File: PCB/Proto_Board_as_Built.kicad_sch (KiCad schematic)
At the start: 17 parts, among them J1 RJ25, J2 RJ45, U1 Pico, U2 LM358

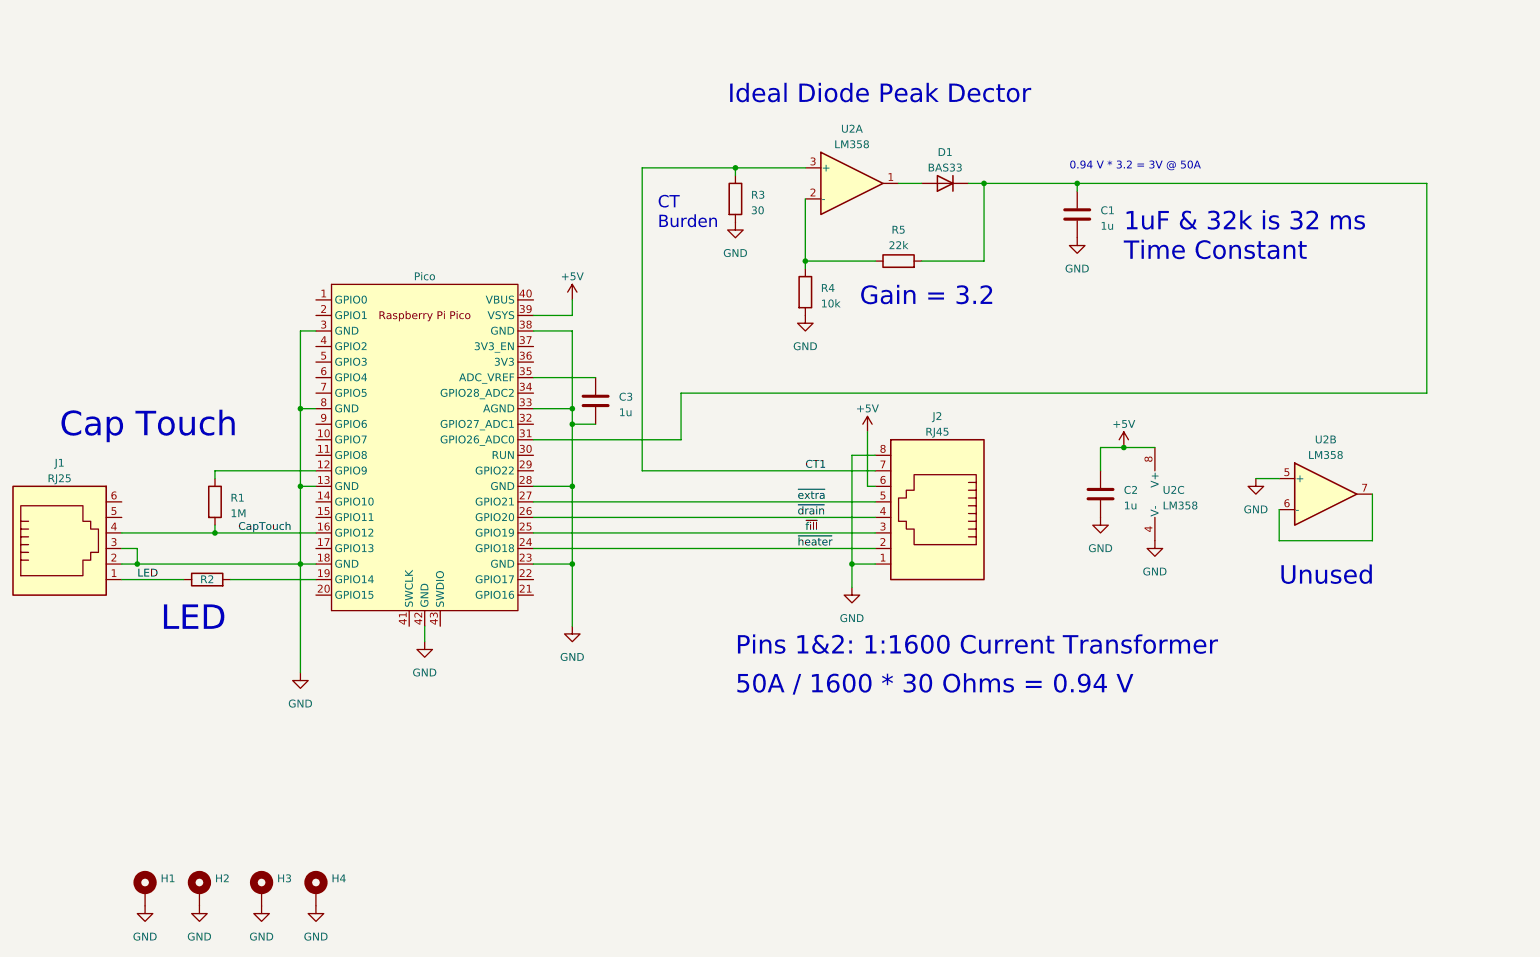
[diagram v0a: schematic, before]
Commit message: pcb updates
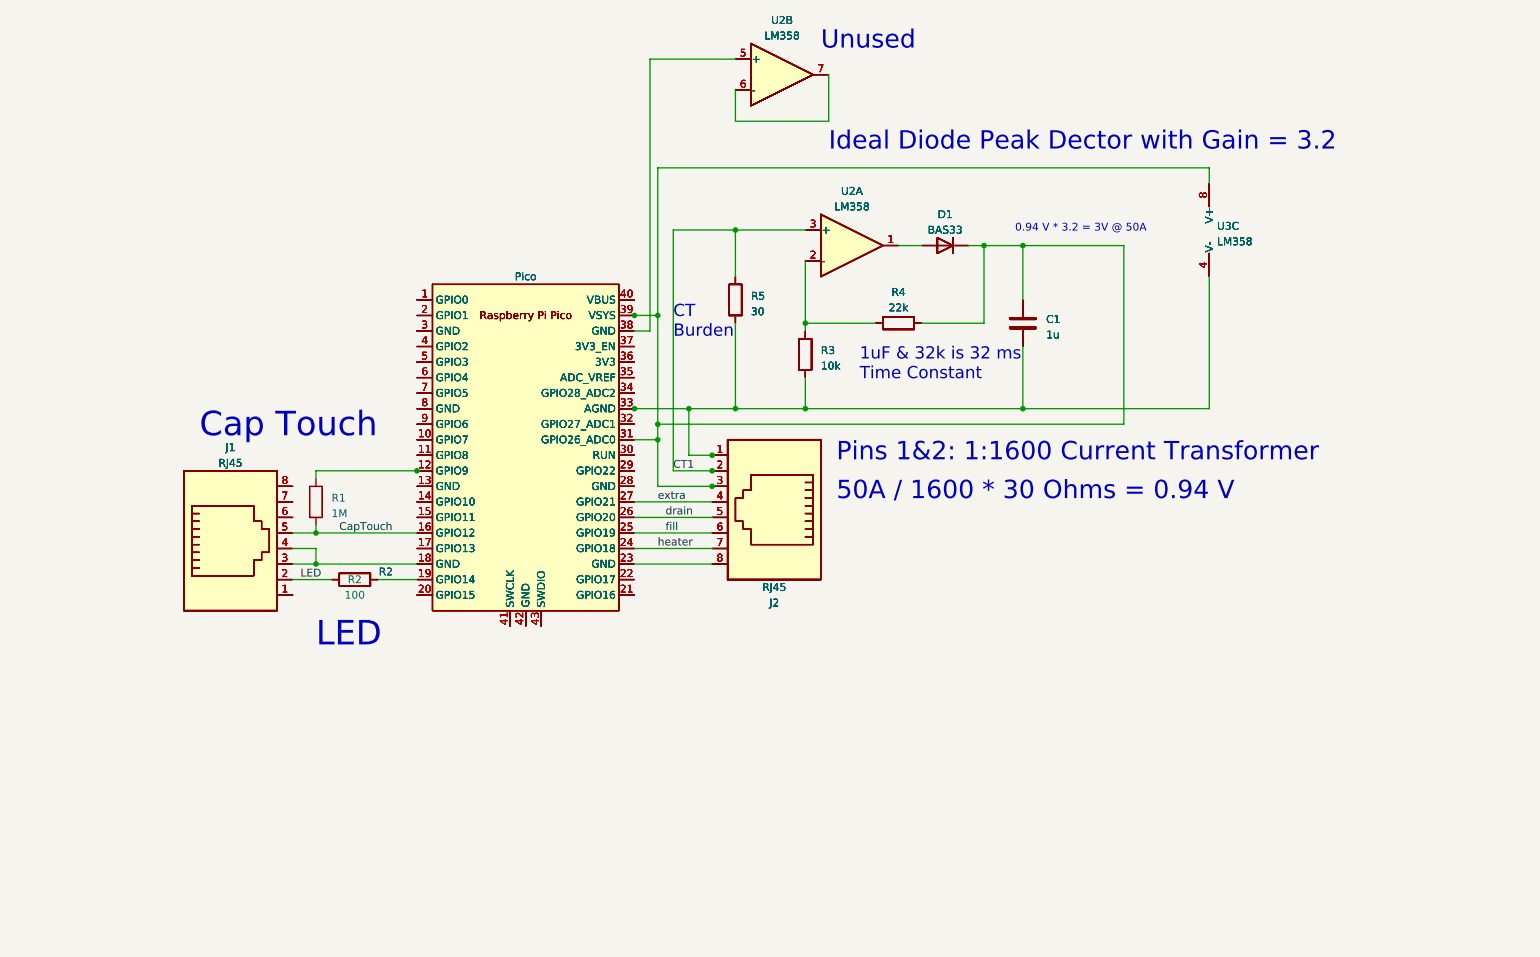
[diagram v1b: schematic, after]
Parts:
- removed C2, C3: 1u, Capacitor_SMD:C_0805_2012Metric_Pad1.18x1.45mm_HandSolder, symbol Device:C
- removed H1, H2, H3, H4: MountingHole_Pad, MountingHole:MountingHole_2.7mm_M2.5_Pad, symbol Mechanical:MountingHole_Pad
- removed J1: RJ25, Connector_RJ:RJ25_Wayconn_MJEA-660X1_Horizontal, symbol Connector:RJ25
- removed J2: RJ45, Connector_RJ:RJ45_Amphenol_54602-x08_Horizontal, symbol Connector:RJ45
- added C1 (x2): 1u, symbol Device:C
- added D1 (x2): BAS33, Diode_THT:D_DO-35_SOD27_P7.62mm_Horizontal, symbol Diode:BAV17
- added J1 (x3), J2 (x3): RJ45, symbol Connector:RJ45
- added R2 (x2): 100, symbol Device:R
- added R3 (x2): 10k, symbol Device:R
- added R4 (x2): 22k, symbol Device:R
- added R5 (x2): 30, symbol Device:R
- added U1 (x2): Pico, MCU_RaspberryPi_and_Boards:RPi_Pico_SMD_TH, symbol MCU_RaspberryPi_and_Boards:Pico
- added U2 (x2), U3 (x2): LM358, symbol Amplifier_Operational:LM358
- C1: footprint Capacitor_SMD:C_0805_2012Metric_Pad1.18x1.45mm_HandSolder -> (none)
- R1, R2: footprint Resistor_SMD:R_0805_2012Metric_Pad1.20x1.40mm_HandSolder -> (none)
- R3: renamed from R4; footprint Resistor_SMD:R_0805_2012Metric_Pad1.20x1.40mm_HandSolder -> (none)
- R4: renamed from R5; footprint Resistor_SMD:R_0805_2012Metric_Pad1.20x1.40mm_HandSolder -> (none)
- R5: renamed from R3; footprint Resistor_SMD:R_0805_2012Metric_Pad1.20x1.40mm_HandSolder -> (none)
- U1: footprint MCU_RaspberryPi_and_Boards:RPi_Pico_SMD -> MCU_RaspberryPi_and_Boards:RPi_Pico_SMD_TH
- U2: footprint Package_DIP:DIP-8_W10.16mm -> (none)
- U3: renamed from U2; footprint Package_DIP:DIP-8_W10.16mm -> (none)
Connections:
- net +5V is gone; now on an unnamed net: U1.39 (VSYS), U3.8 (V+)
- net CT1: now also J2.2, J2.2, J2.2, R5.1, R5.1, U2.3 (+), U2.3 (+)
- net CapTouch: now also J1.5, J1.5, J1.5, U1.16 (GPIO12), U1.16 (GPIO12)
- net LED: now also J1.2, J1.2, J1.2, R2.1, R2.1
- net at C1.1, D1.1 (K), R4.2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: now also C1.1, C1.1, D1.1 (K), D1.1 (K), J2.3, J2.3, J2.3, R4.2, R4.2, U1.31 (GPIO26_ADC0), U1.31 (GPIO26_ADC0), U1.39 (VSYS), U1.39 (VSYS), U3.8 (V+), U3.8 (V+)
- net at U1.1 (GPIO0): now also U1.1 (GPIO0), U1.1 (GPIO0)
- net at U1.10 (GPIO7): now also U1.10 (GPIO7), U1.10 (GPIO7)
- net at U1.11 (GPIO8): now also U1.11 (GPIO8), U1.11 (GPIO8)
- net at R1.1, U1.12 (GPIO9): now also U1.12 (GPIO9), U1.12 (GPIO9)
- net at U1.14 (GPIO10): now also U1.14 (GPIO10), U1.14 (GPIO10)
- net at U1.15 (GPIO11): now also U1.15 (GPIO11), U1.15 (GPIO11)
- net at U1.17 (GPIO13): now also U1.17 (GPIO13), U1.17 (GPIO13)
- net at R2.2, U1.19 (GPIO14): now also R2.2, R2.2, U1.19 (GPIO14), U1.19 (GPIO14)
- net at U1.2 (GPIO1): now also U1.2 (GPIO1), U1.2 (GPIO1)
- net at U1.20 (GPIO15): now also U1.20 (GPIO15), U1.20 (GPIO15)
- net at U1.21 (GPIO16): now also U1.21 (GPIO16), U1.21 (GPIO16)
- net at U1.22 (GPIO17): now also U1.22 (GPIO17), U1.22 (GPIO17)
- net at U1.29 (GPIO22): now also U1.29 (GPIO22), U1.29 (GPIO22)
- net at U1.30 (RUN): now also U1.30 (RUN), U1.30 (RUN)
- net at U1.32 (GPIO27_ADC1): now also U1.32 (GPIO27_ADC1), U1.32 (GPIO27_ADC1)
- net at U1.34 (GPIO28_ADC2): now also U1.34 (GPIO28_ADC2), U1.34 (GPIO28_ADC2)
- net at U1.35 (ADC_VREF): now also U1.35 (ADC_VREF), U1.35 (ADC_VREF)
- net at U1.36 (3V3): now also U1.36 (3V3), U1.36 (3V3)
- net at U1.37 (3V3_EN): now also U1.37 (3V3_EN), U1.37 (3V3_EN)
- net at U1.4 (GPIO2): now also U1.4 (GPIO2), U1.4 (GPIO2)
- net at U1.40 (VBUS): now also U1.40 (VBUS), U1.40 (VBUS)
- net at U1.41 (SWCLK): now also U1.41 (SWCLK), U1.41 (SWCLK)
- net at U1.43 (SWDIO): now also U1.43 (SWDIO), U1.43 (SWDIO)
- net at U1.5 (GPIO3): now also U1.5 (GPIO3), U1.5 (GPIO3)
- net at U1.6 (GPIO4): now also U1.6 (GPIO4), U1.6 (GPIO4)
- net at U1.7 (GPIO5): now also U1.7 (GPIO5), U1.7 (GPIO5)
- net at U1.9 (GPIO6): now also U1.9 (GPIO6), U1.9 (GPIO6)
- net at D1.2 (A), U2.1: now also D1.2 (A), D1.2 (A), U2.1, U2.1
- net at R3.1, R4.1, U2.2 (-): now also R3.1, R3.1, R4.1, R4.1, U2.2 (-), U2.2 (-)
- net at U2.6 (-), U2.7: now also U2.6 (-), U2.6 (-), U2.7, U2.7
- removed net GND: C1.2, R3.2, R5.2, U1.13 (GND), U1.18 (GND), U1.23 (GND), U1.28 (GND), U1.3 (GND), U1.33 (AGND), U1.38 (GND), U1.42 (GND), U1.8 (GND), U2.5 (+), U3.4 (V-)
- net ~{drain} renamed drain
- net drain: now also J2.5, J2.5, J2.5, U1.26 (GPIO20), U1.26 (GPIO20)
- net ~{extra} renamed extra
- net extra: now also J2.4, J2.4, J2.4, U1.27 (GPIO21), U1.27 (GPIO21)
- net ~{fill} renamed fill
- net fill: now also J2.6, J2.6, J2.6, U1.25 (GPIO19), U1.25 (GPIO19)
- net ~{heater} renamed heater
- net heater: now also J2.7, J2.7, J2.7, U1.24 (GPIO18), U1.24 (GPIO18)
- new net: C1.2, C1.2, C1.2, J2.1, J2.1, J2.1, R3.2, R3.2, R3.2, R5.2, R5.2, R5.2, U1.33 (AGND), U1.33 (AGND), U1.33 (AGND), U3.4 (V-), U3.4 (V-), U3.4 (V-)
- new net: J2.8, J2.8, J2.8, U1.23 (GND), U1.23 (GND), U1.23 (GND)
- new net: J1.1, J1.1, J1.1
- new net: J1.3, J1.3, J1.3, J1.4, J1.4, J1.4, U1.18 (GND), U1.18 (GND), U1.18 (GND)
- new net: J1.6, J1.6, J1.6
- new net: J1.7, J1.7, J1.7
- new net: J1.8, J1.8, J1.8
- new net: U1.13 (GND), U1.13 (GND), U1.13 (GND)
- new net: U1.28 (GND), U1.28 (GND), U1.28 (GND)
- new net: U1.3 (GND), U1.3 (GND), U1.3 (GND)
- new net: U1.38 (GND), U1.38 (GND), U1.38 (GND), U2.5 (+), U2.5 (+), U2.5 (+)
- new net: U1.42 (GND), U1.42 (GND), U1.42 (GND)
- new net: U1.8 (GND), U1.8 (GND), U1.8 (GND)
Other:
- note added: "Ideal Diode Peak Dector with Gain = 3.2"
- note removed: "Gain = 3.2"
- note removed: "Ideal Diode Peak Dector"
- moved on the sheet: C1, D1, R1, R2, R3, R4, R5, U2A, U2B, U3C
